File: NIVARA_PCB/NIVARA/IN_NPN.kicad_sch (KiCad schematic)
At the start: 14 parts, among them U2 AT3H4A-CUH-S, U4 AT3H4A-CUH-S

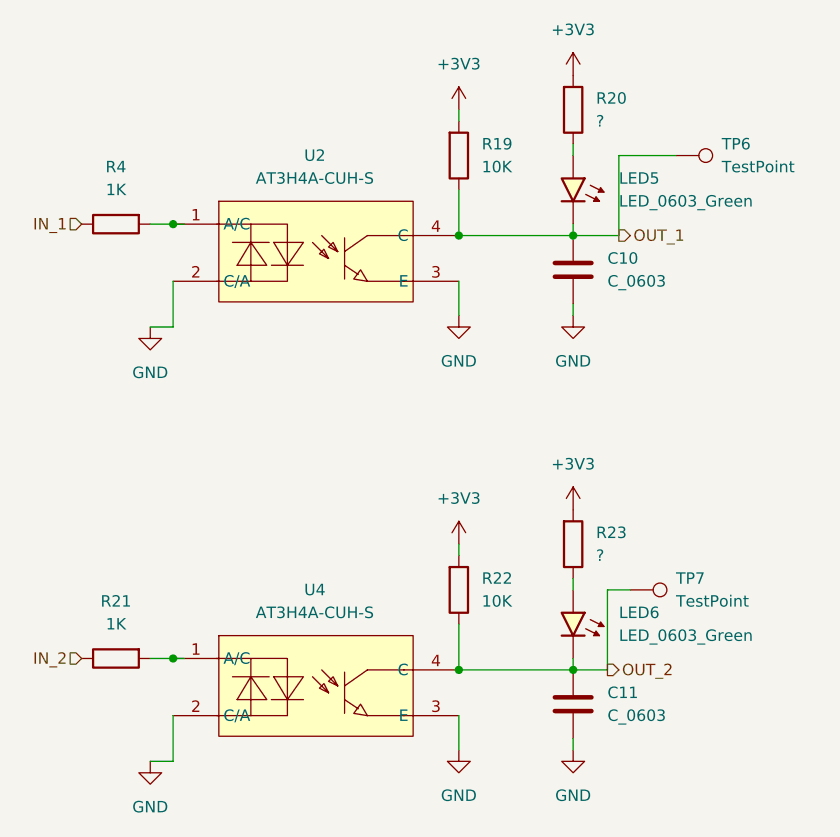
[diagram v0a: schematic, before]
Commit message: avance
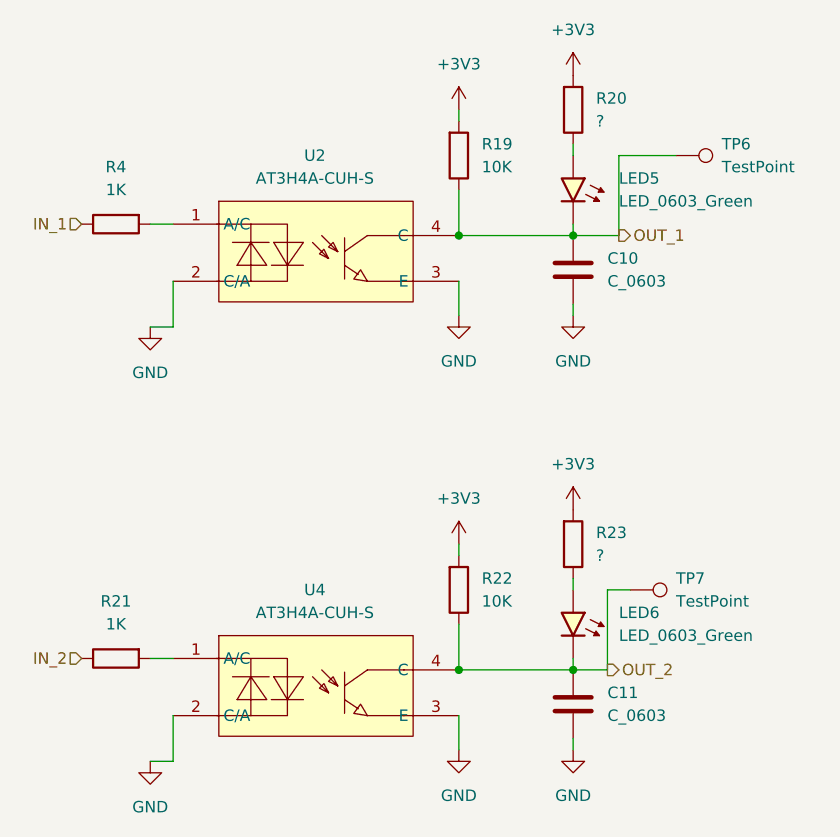
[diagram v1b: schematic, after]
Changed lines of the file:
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@@
-	)
-	(junction
-		(at 119.38 64.77)
-		(diameter 0)
-		(color 0 0 0 0)
 	)
 	(junction
@@
 		(color 0 0 0 0)
 	)
-	(junction
-		(at 119.38 113.03)
-		(diameter 0)
-		(color 0 0 0 0)
-	)
 	(wire
 		(pts
 			(xy 163.83 123.19) (xy 163.83 121.92)
-		)
-		(stroke
-			(width 0)
-			(type default)
-		)
-	)
-	(wire
-		(pts
-			(xy 119.38 64.77) (xy 120.65 64.77)
 		)
 		(stroke
@@
 	(wire
 		(pts
-			(xy 116.84 113.03) (xy 119.38 113.03)
-		)
-		(stroke
-			(width 0)
-			(type default)
-		)
-	)
-	(wire
-		(pts
 			(xy 151.13 52.07) (xy 151.13 53.34)
 		)
@@
 		(pts
 			(xy 151.13 74.93) (xy 151.13 71.12)
-		)
-		(stroke
-			(width 0)
-			(type default)
-		)
-	)
-	(wire
-		(pts
-			(xy 119.38 113.03) (xy 120.65 113.03)
 		)
 		(stroke
@@
 		)
 		(stroke
+			(width 0)
+			(type default)
+		)
+	)
+	(wire
+		(pts
+			(xy 116.84 113.03) (xy 119.38 113.03)
+		)
+		(stroke
